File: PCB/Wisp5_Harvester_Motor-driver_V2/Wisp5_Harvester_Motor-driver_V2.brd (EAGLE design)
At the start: 30 x 30 mm, 29 parts, among them M1 PINHEAD_PINHD-1X2-1.27MM, M2 PINHEAD_PINHD-1X2-1.27MM, U1 BQ25570

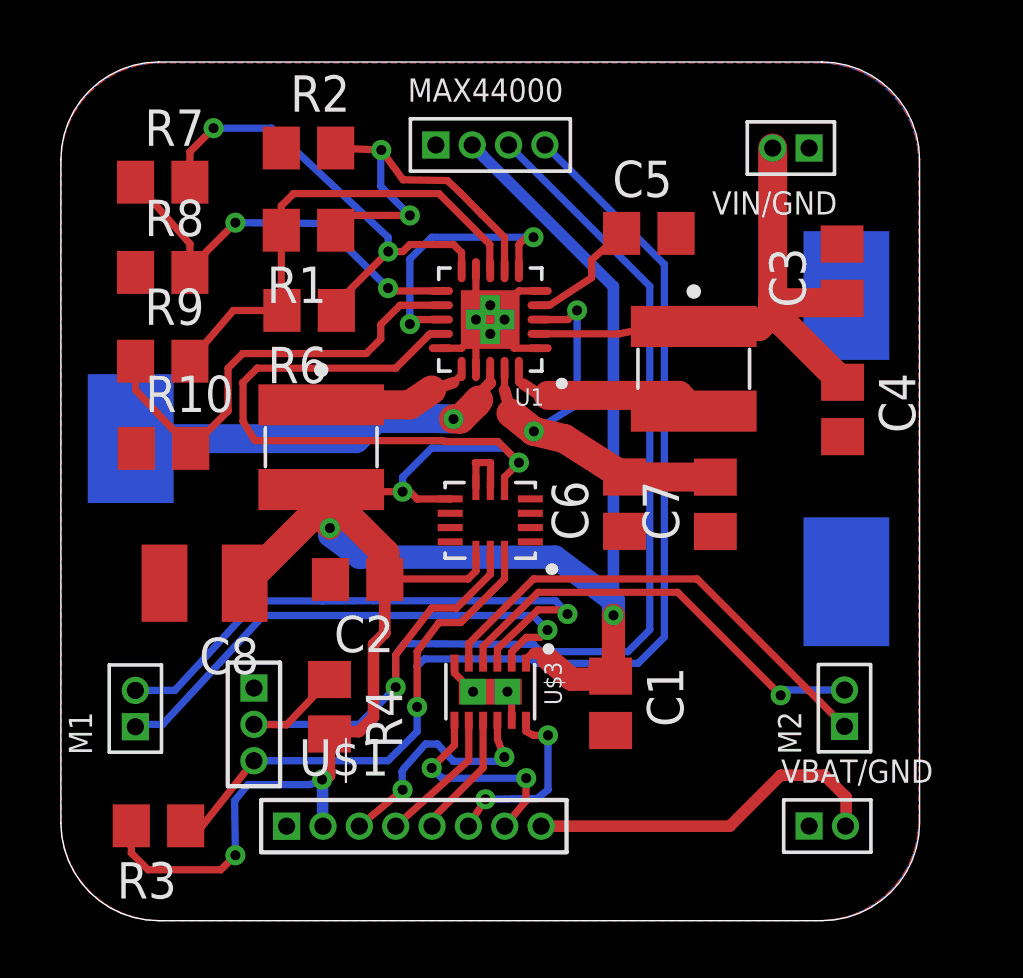
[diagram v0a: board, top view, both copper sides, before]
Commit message: Fix the naming on the pcb and of the parts!
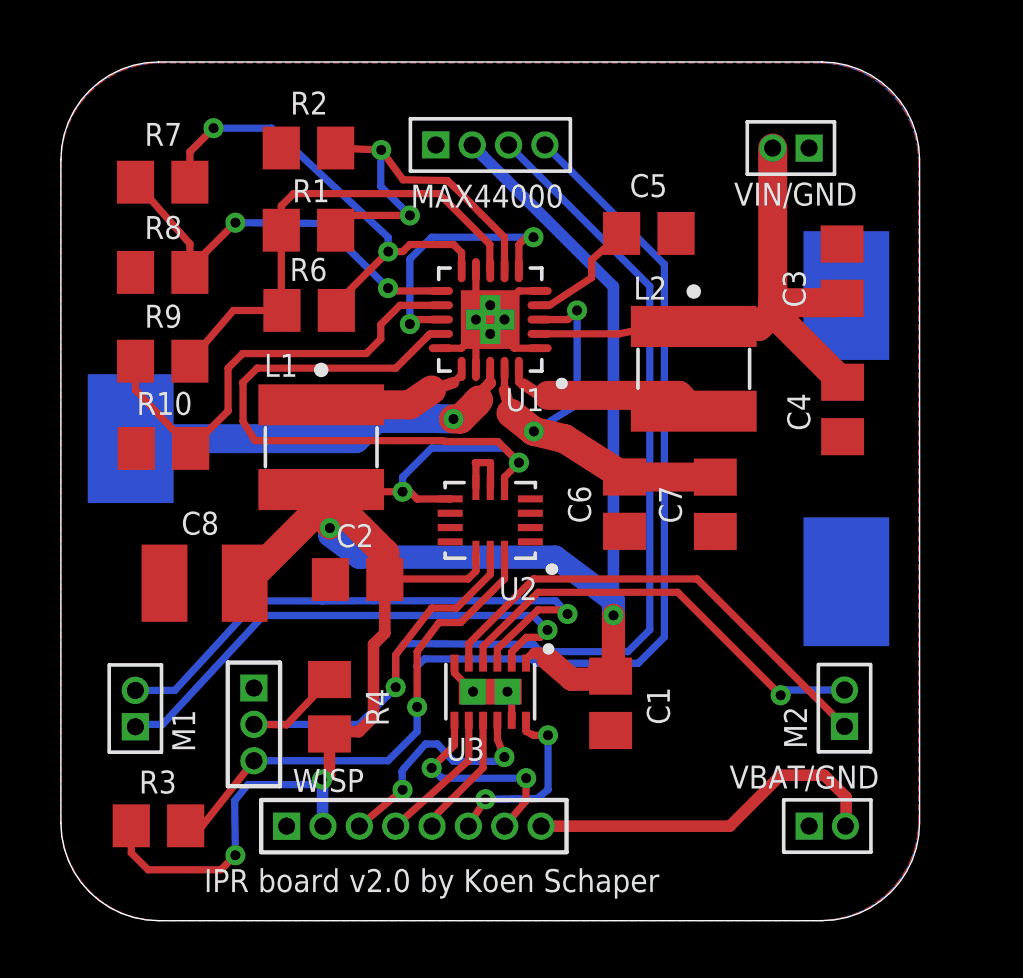
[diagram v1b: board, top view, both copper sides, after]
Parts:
- L1: value 22uH -> (none)
- L2: value 10uH -> (none)
- renumbered U$1 to WISP, U$2 to U2, U$3 to U3
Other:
- board text added: "IPR board v2.0 by Koen Schaper"
- board text added: "L1"
- board text added: "L2"
- board text added: "U2"
